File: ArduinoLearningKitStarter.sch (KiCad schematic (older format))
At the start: 80 parts, among them J1 USB_OTG, J2 CONN_01X08, J3 CONN_01X06, J4 CONN_01X08, J5 CONN_01X10, J6 CONN_01X04, J7 CONN_01X04, J8 CONN_01X02, SW1 SW_PUSH, SW2 SW_PUSH, SW3 SW_PUSH, U1 arduino_nano, U2 arduino_uno, U3 ESP32-DEVKIT-C

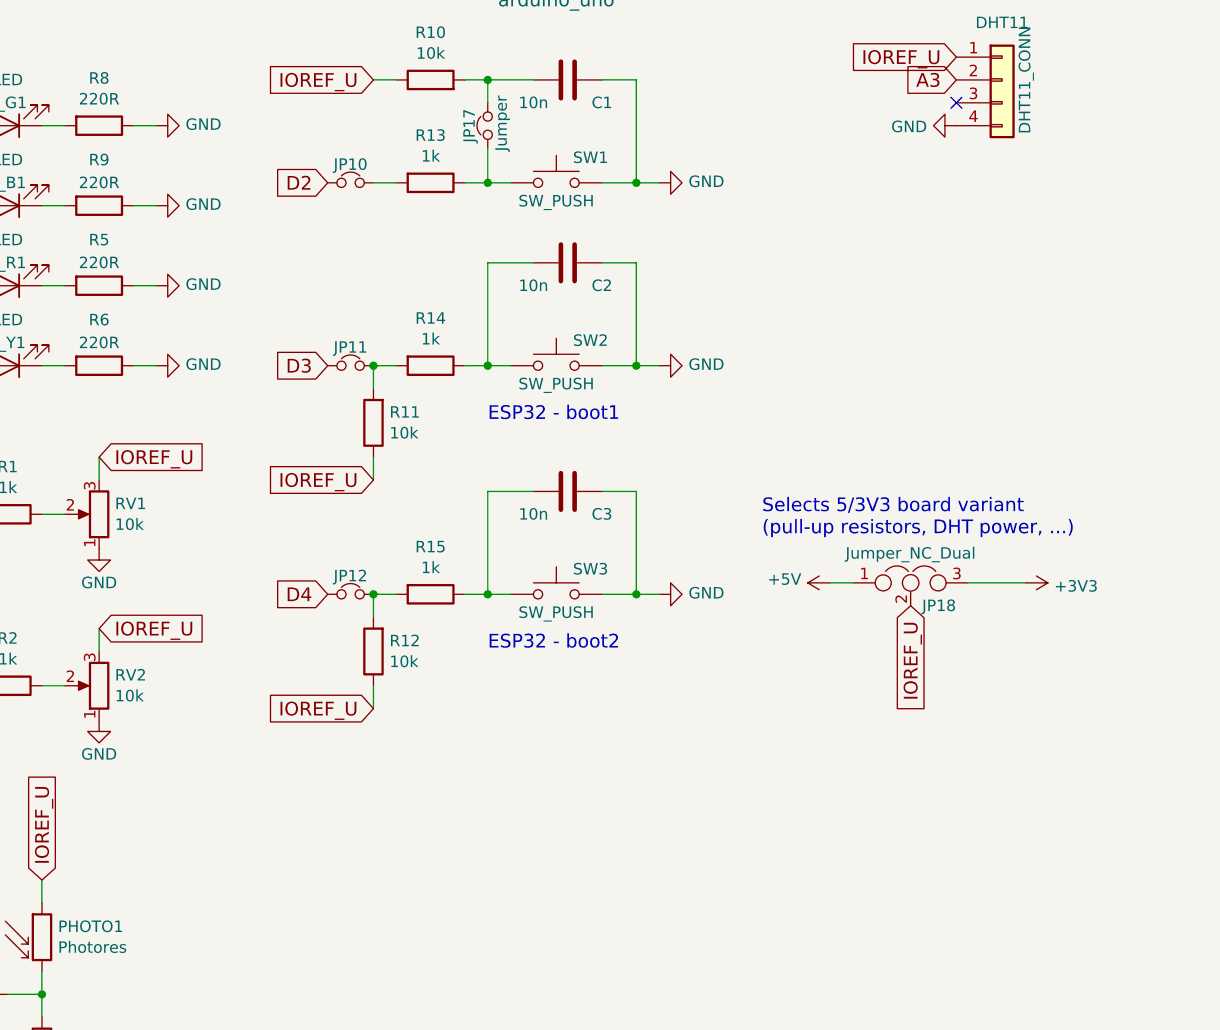
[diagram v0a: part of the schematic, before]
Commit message: Suggest new layout
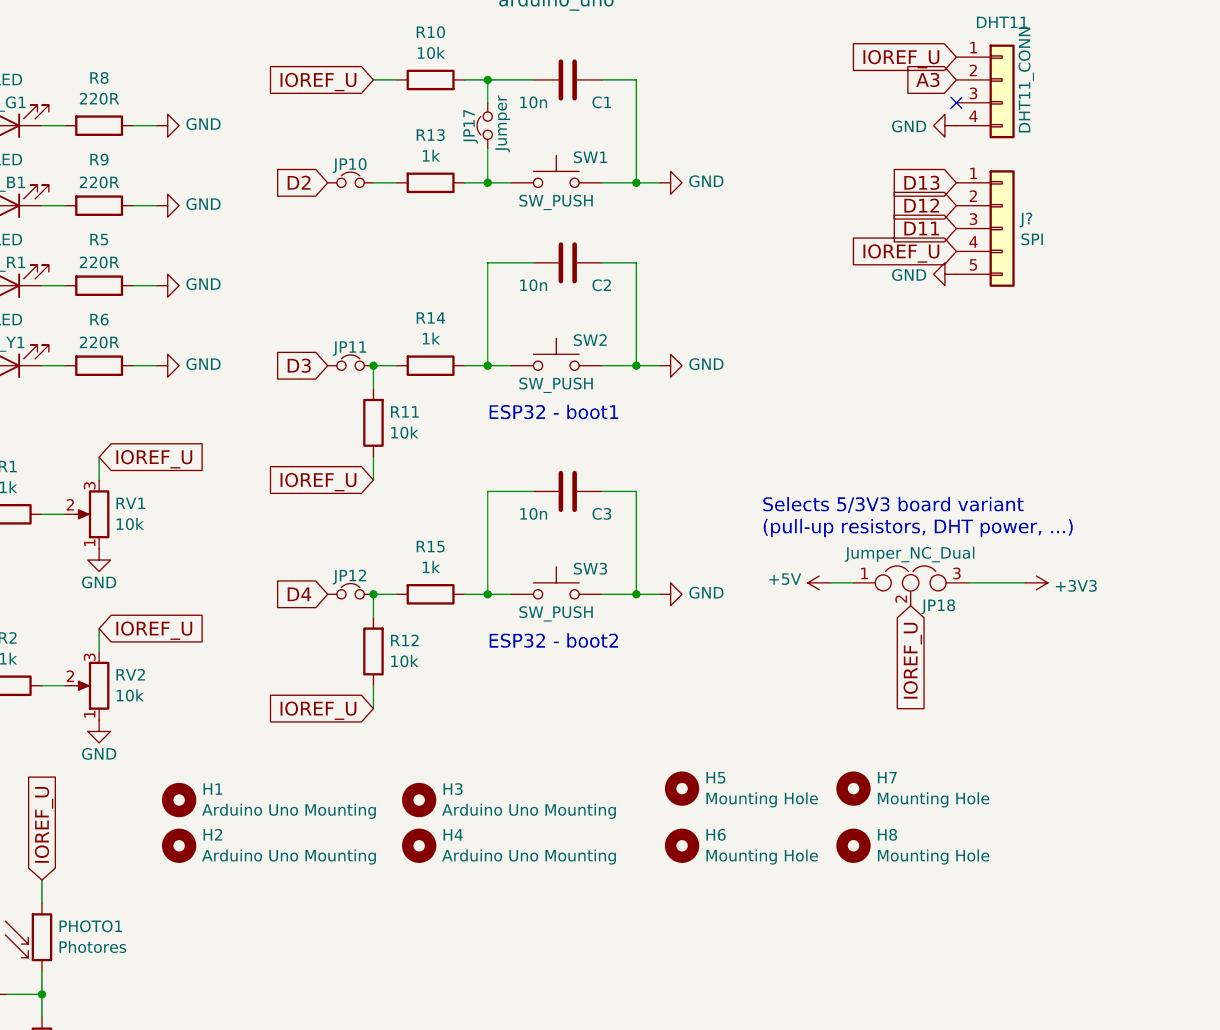
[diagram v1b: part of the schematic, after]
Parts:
- added H1, H2, H3, H4: Arduino Uno Mounting, MountingHole:MountingHole_2.2mm_M2, symbol Mechanical:MountingHole
- added H5, H6, H7, H8: Mounting Hole, MountingHole:MountingHole_2.2mm_M2, symbol Mechanical:MountingHole
- added J?: SPI, Connector_PinHeader_2.54mm:PinHeader_1x05_P2.54mm_Horizontal, symbol Connector_Generic:Conn_01x05
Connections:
- net D11: now also J?.3 (Pin_3)
- net D12: now also J?.2 (Pin_2)
- net D13: now also J?.1 (Pin_1)
- net GND: now also J?.5 (Pin_5)
- net IOREF_U: now also J?.4 (Pin_4)
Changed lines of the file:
@@
 Wire Wire Line
 	6050 3250 6150 3250
+$Comp
+L Mechanical:MountingHole H2
+U 1 1 5C1DAAED
+P 7050 6400
+F 0 "H2" H 7150 6446 50  0000 L CNN
+F 1 "Arduino Uno Mounting" H 7150 6355 50  0000 L CNN
+F 2 "MountingHole:MountingHole_2.2mm_M2" H 7050 6400 50  0001 C CNN
+F 3 "~" H 7050 6400 50  0001 C CNN
+	1    7050 6400
+	1    0    0    -1
+$EndComp
+$Comp
+L Mechanical:MountingHole H1
+U 1 1 5C1DB830
+P 7050 6200
+F 0 "H1" H 7150 6246 50  0000 L CNN
+F 1 "Arduino Uno Mounting" H 7150 6155 50  0000 L CNN
+F 2 "MountingHole:MountingHole_2.2mm_M2" H 7050 6200 50  0001 C CNN
+F 3 "~" H 7050 6200 50  0001 C CNN
+	1    7050 6200
+	1    0    0    -1
+$EndComp
+$Comp
+L Mechanical:MountingHole H3
+U 1 1 5C1DB922
+P 8100 6200
+F 0 "H3" H 8200 6246 50  0000 L CNN
+F 1 "Arduino Uno Mounting" H 8200 6155 50  0000 L CNN
+F 2 "MountingHole:MountingHole_2.2mm_M2" H 8100 6200 50  0001 C CNN
+F 3 "~" H 8100 6200 50  0001 C CNN
+	1    8100 6200
+	1    0    0    -1
+$EndComp
+$Comp
+L Mechanical:MountingHole H4
+U 1 1 5C1DBA12
+P 8100 6400
+F 0 "H4" H 8200 6446 50  0000 L CNN
+F 1 "Arduino Uno Mounting" H 8200 6355 50  0000 L CNN
+F 2 "MountingHole:MountingHole_2.2mm_M2" H 8100 6400 50  0001 C CNN
+F 3 "~" H 8100 6400 50  0001 C CNN
+	1    8100 6400
+	1    0    0    -1
+$EndComp
+$Comp
+L Mechanical:MountingHole H5
+U 1 1 5C1E65A4
+P 9250 6150
+F 0 "H5" H 9350 6196 50  0000 L CNN
+F 1 "Mounting Hole" H 9350 6105 50  0000 L CNN
+F 2 "MountingHole:MountingHole_2.2mm_M2" H 9250 6150 50  0001 C CNN
+F 3 "~" H 9250 6150 50  0001 C CNN
+	1    9250 6150
+	1    0    0    -1
+$EndComp
+$Comp
+L Mechanical:MountingHole H6
+U 1 1 5C1E68AB
+P 9250 6400
+F 0 "H6" H 9350 6446 50  0000 L CNN
+F 1 "Mounting Hole" H 9350 6355 50  0000 L CNN
+F 2 "MountingHole:MountingHole_2.2mm_M2" H 9250 6400 50  0001 C CNN
+F 3 "~" H 9250 6400 50  0001 C CNN
+	1    9250 6400
+	1    0    0    -1
+$EndComp
+$Comp
+L Mechanical:MountingHole H7
+U 1 1 5C1E6975
+P 10000 6150
+F 0 "H7" H 10100 6196 50  0000 L CNN
+F 1 "Mounting Hole" H 10100 6105 50  0000 L CNN
+F 2 "MountingHole:MountingHole_2.2mm_M2" H 10000 6150 50  0001 C CNN
+F 3 "~" H 10000 6150 50  0001 C CNN
+	1    10000 6150
+	1    0    0    -1
+$EndComp
+$Comp
+L Mechanical:MountingHole H8
+U 1 1 5C1E6A5D
+P 10000 6400
+F 0 "H8" H 10100 6446 50  0000 L CNN
+F 1 "Mounting Hole" H 10100 6355 50  0000 L CNN
+F 2 "MountingHole:MountingHole_2.2mm_M2" H 10000 6400 50  0001 C CNN
+F 3 "~" H 10000 6400 50  0001 C CNN
+	1    10000 6400
+	1    0    0    -1
+$EndComp
+$Comp
+L Connector_Generic:Conn_01x05 J?
+U 1 1 5C1EA8A1
+P 10650 3700
+F 0 "J?" H 10730 3742 50  0000 L CNN
+F 1 "SPI" H 10730 3651 50  0000 L CNN
+F 2 "Connector_PinHeader_2.54mm:PinHeader_1x05_P2.54mm_Horizontal" H 10650 3700 50  0001 C CNN
+F 3 "~" H 10650 3700 50  0001 C CNN
+	1    10650 3700
+	1    0    0    -1
+$EndComp
+$Comp
+L ArduinoLearningKitStarter:GND #PWR?
+U 1 1 5C1EAB4C
+P 10450 3900
+F 0 "#PWR?" H 10450 3650 50  0001 C CNN
+F 1 "GND" V 10455 3772 50  0000 R CNN
+F 2 "" H 10450 3900 50  0000 C CNN
+F 3 "" H 10450 3900 50  0000 C CNN
+	1    10450 3900
+	0    1    1    0
+$EndComp
+Text GLabel 10450 3800 0    60   Input ~ 0
+IOREF_U
+Text GLabel 10450 3600 0    60   Input ~ 0
+D12
+Text GLabel 10450 3500 0    60   Input ~ 0
+D13
+Text GLabel 10450 3700 0    60   Input ~ 0
+D11
 $EndSCHEMATC
